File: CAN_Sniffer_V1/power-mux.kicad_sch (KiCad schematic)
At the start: 7 parts, among them IC1 TPS2121RUXR

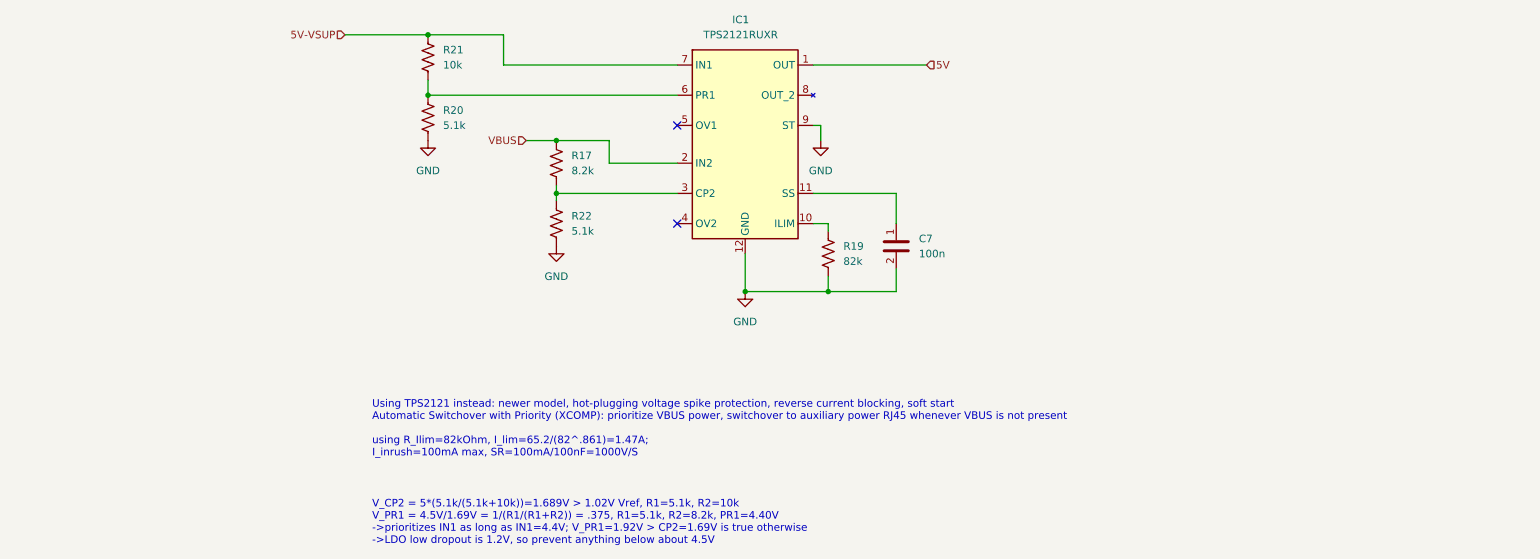
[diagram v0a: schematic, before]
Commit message: iteration 2 routing
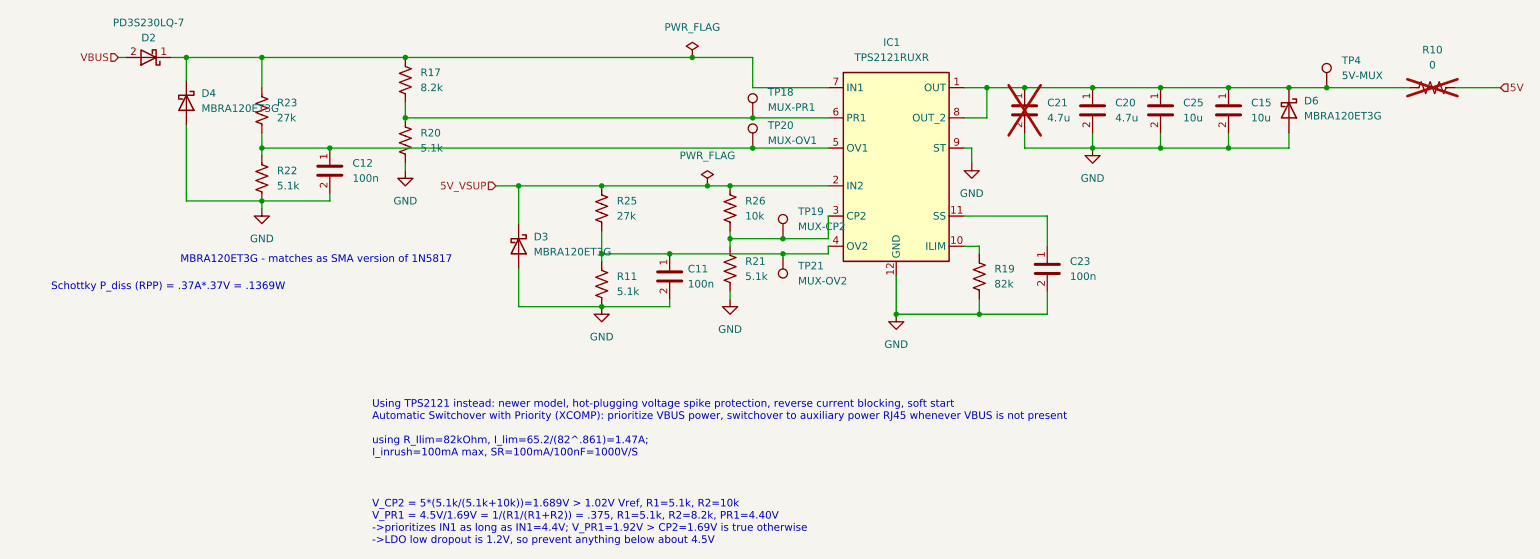
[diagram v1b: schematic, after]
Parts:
- removed C7: 100n, Capacitor_SMD:C_0402_1005Metric_Pad0.74x0.62mm_HandSolder, symbol bfr_capacitors:CL05B104KB54PNC
- removed R20, R22: 5.1k, Resistor_SMD:R_0402_1005Metric_Pad0.72x0.64mm_HandSolder, symbol bfr_resistors:RMCF0402FT5K10
- removed R21: 10k, Resistor_SMD:R_0402_1005Metric_Pad0.72x0.64mm_HandSolder, symbol bfr_resistors:RMCF0402FT10K0
- added C11, C12: 100n, Capacitor_SMD:C_0402_1005Metric_Pad0.74x0.62mm_HandSolder, symbol bfr_capacitors:CL05B104KB54PNC
- added C15, C25: 10u, Capacitor_SMD:C_0603_1608Metric_Pad1.08x0.95mm_HandSolder, symbol bfr_capacitors:CL10A106MA8NRNC
- added C20, C21: 4.7u, Capacitor_SMD:C_0603_1608Metric_Pad1.08x0.95mm_HandSolder, symbol bfr_capacitors:CL10A475KO8NNNC
- added C23: 100n, Capacitor_SMD:C_0603_1608Metric_Pad1.08x0.95mm_HandSolder, symbol bfr_capacitors:06035C104KAT2A
- added D2: PD3S230LQ-7, PD3S230LQ-7:PD3S230LQ7, symbol PD3S230LQ-7:PD3S230LQ-7
- added D3, D4, D6: MBRA120ET3G, Diode_SMD:D_SMA_Handsoldering, symbol Diode:1N5817
- added R10: 0, Resistor_SMD:R_0805_2012Metric_Pad1.20x1.40mm_HandSolder, symbol bfr_resistors:RMCF0805ZT0R00
- added R11, R20, R21, R22: 5.1k, Resistor_SMD:R_0603_1608Metric_Pad0.98x0.95mm_HandSolder, symbol bfr_resistors:RMCF0603FT5K10
- added R23, R25: 27k, Resistor_SMD:R_0603_1608Metric_Pad0.98x0.95mm_HandSolder, symbol bfr_resistors:RMCF0603FT27K0
- added R26: 10k, Resistor_SMD:R_0603_1608Metric_Pad0.98x0.95mm_HandSolder, symbol bfr_resistors:RMCF0603FT10K0
- added TP18: MUX-PR1, TestPoint:TestPoint_Pad_D1.0mm, symbol Connector:TestPoint
- added TP19: MUX-CP2, TestPoint:TestPoint_Pad_D1.0mm, symbol Connector:TestPoint
- added TP20: MUX-OV1, TestPoint:TestPoint_Pad_D1.0mm, symbol Connector:TestPoint
- added TP21: MUX-OV2, TestPoint:TestPoint_Pad_D1.0mm, symbol Connector:TestPoint
- added TP4: 5V-MUX, TestPoint:TestPoint_Pad_D1.0mm, symbol Connector:TestPoint
- IC1: JLC link (none) -> https://jlcpcb.com/partdetail/TexasInstruments-TPS2121RUXR/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
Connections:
- net 5V: now also R10.2; no longer IC1.1 (OUT)
- net GND: now also C11.2, C12.2, C15.2, C20.2, C21.2, C23.2, C25.2, D3.2 (A), D4.2 (A), D6.2 (A), R11.1, R20.1, R21.1, R22.1
- net VBUS: now also D2.2 (A); no longer IC1.2 (IN2), R17.2
- net at IC1.11 (SS): now also C23.1
- net at IC1.3 (CP2): now also R21.2, R26.1, TP19.1; no longer R17.1
- net at IC1.4 (OV2): now also C11.1, R11.2, R25.1, TP21.1
- net at IC1.5 (OV1): now also C12.1, R22.2, R23.1, TP20.1
- net at IC1.6 (PR1): now also R17.1, R20.2, TP18.1
- net at IC1.8 (OUT_2): now also IC1.1 (OUT), C15.1, C20.1, C21.1, C25.1, D6.1 (K), R10.1, TP4.1
- net 5V-VSUP: no longer names the net of IC1.7 (IN1)
- net 5V-VSUP: now also R17.2, D2.1 (K), D4.1 (K), R23.2
- new net 5V_VSUP: D3.1 (K), IC1.2 (IN2), R25.2, R26.2
- no-connect marks 2 -> 0
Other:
- note added: "MBRA120ET3G - matches as SMA version of 1N5817"
- note added: "Schottky P_diss (RPP) = .37A*.37V = .1369W"
- moved on the sheet: R17, R19

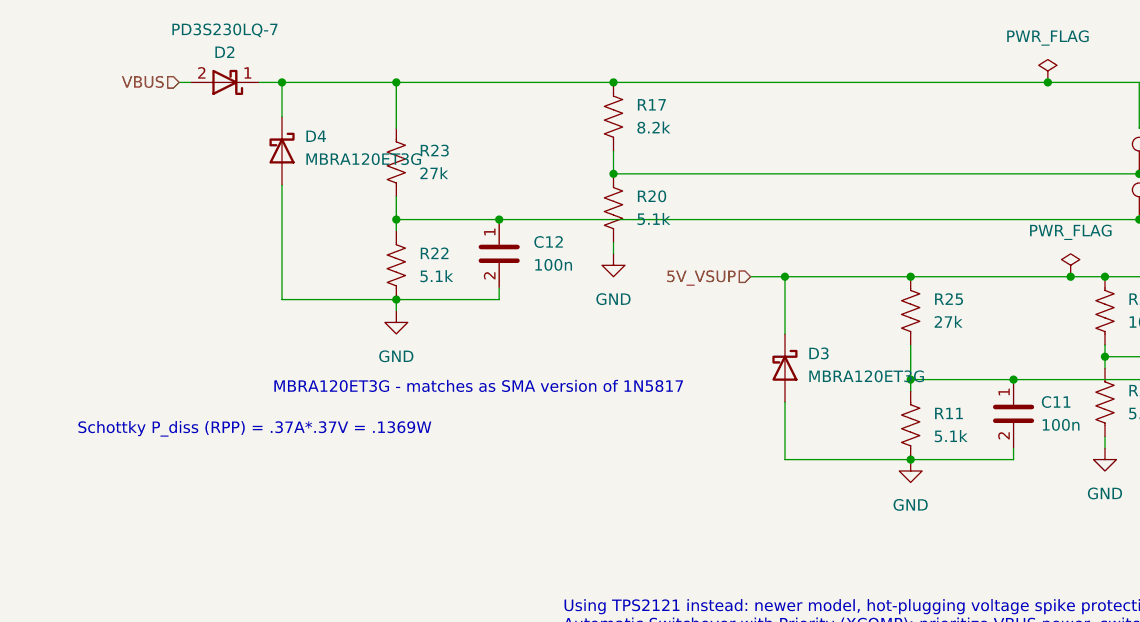
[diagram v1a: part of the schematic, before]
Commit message: sync changes
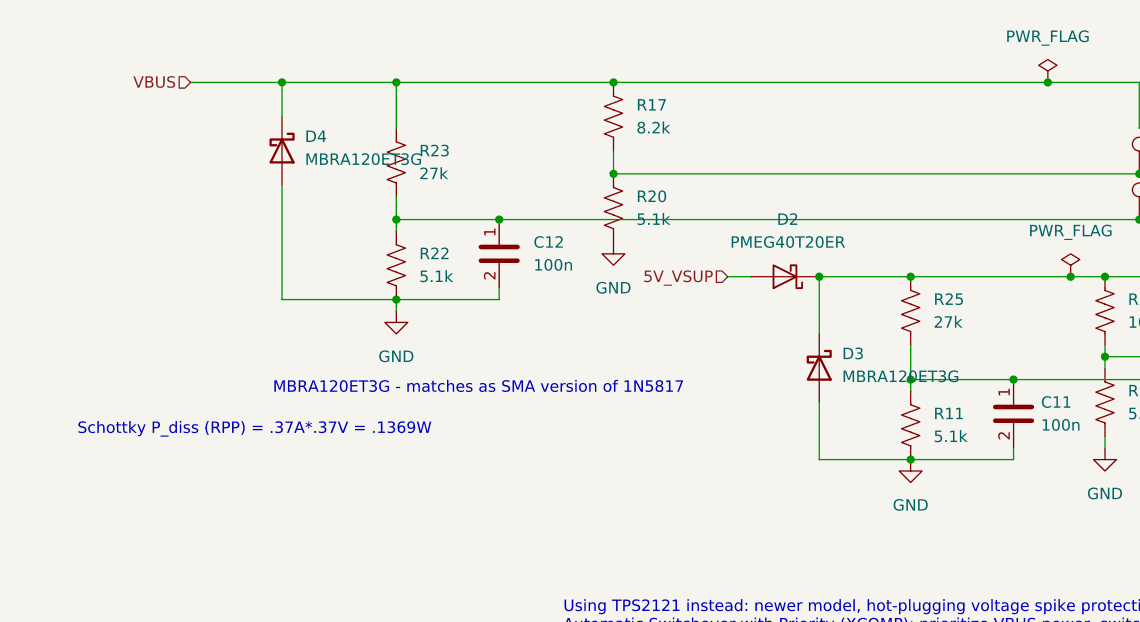
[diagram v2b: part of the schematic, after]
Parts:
- removed D2: PD3S230LQ-7, PD3S230LQ-7:PD3S230LQ7, symbol PD3S230LQ-7:PD3S230LQ-7
- added D2: PMEG40T20ER, Diode_SMD:Nexperia_CFP3_SOD-123W, symbol Diode:PMEG40T20ER
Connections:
- net 5V_VSUP: now also D2.2 (A); no longer D3.1 (K), IC1.2 (IN2), R25.2, R26.2
- net VBUS: now also D4.1 (K), IC1.7 (IN1), R17.2, R23.2
- new net: D2.1 (K), D3.1 (K), IC1.2 (IN2), R25.2, R26.2
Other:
- moved on the sheet: D3
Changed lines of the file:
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@@
 	)
 	(junction
+		(at 105.41 83.82)
+		(diameter 0)
+		(color 0 0 0 0)
+	)
+	(junction
 		(at 180.34 67.31)
 		(diameter 0)
@@
 	)
 	(junction
-		(at 101.6 83.82)
-		(diameter 0)
-		(color 0 0 0 0)
-	)
-	(junction
 		(at 69.85 77.47)
 		(diameter 0)
@@
 	(wire
 		(pts
-			(xy 43.18 62.23) (xy 45.72 62.23)
-		)
-		(stroke
-			(width 0)
-			(type default)
-		)
-	)
-	(wire
-		(pts
 			(xy 130.81 62.23) (xy 140.97 62.23)
 		)
@@
 	(wire
 		(pts
-			(xy 101.6 83.82) (xy 101.6 90.17)
+			(xy 105.41 83.82) (xy 105.41 90.17)
 		)
 		(stroke
@@
 	(wire
 		(pts
-			(xy 82.55 81.28) (xy 82.55 80.01)
-		)
-		(stroke
-			(width 0)
-			(type default)
-		)
-	)
-	(wire
-		(pts
 			(xy 82.55 62.23) (xy 130.81 62.23)
 		)
@@
 	(wire
 		(pts
-			(xy 101.6 104.14) (xy 115.57 104.14)
+			(xy 105.41 104.14) (xy 115.57 104.14)
 		)
 		(stroke
@@
 	(wire
 		(pts
-			(xy 101.6 97.79) (xy 101.6 104.14)
+			(xy 105.41 97.79) (xy 105.41 104.14)
 		)
 		(stroke
@@
 	(wire
 		(pts
-			(xy 101.6 83.82) (xy 115.57 83.82)
-		)
-		(stroke
-			(width 0)
-			(type default)
-		)
-	)
-	(wire
-		(pts
 			(xy 179.07 105.41) (xy 179.07 102.87)
 		)
@@
 	(wire
 		(pts
-			(xy 97.79 83.82) (xy 101.6 83.82)
+			(xy 95.25 83.82) (xy 97.79 83.82)
 		)
 		(stroke
@@
 	(wire
 		(pts
-			(xy 34.29 62.23) (xy 35.56 62.23)
+			(xy 35.56 62.23) (xy 45.72 62.23)
 		)
 		(stroke
@@
 	(wire
 		(pts
+			(xy 105.41 83.82) (xy 115.57 83.82)
+		)
+		(stroke
+			(width 0)
+			(type default)
+		)
+	)
+	(wire
+		(pts
 			(xy 140.97 67.31) (xy 153.67 67.31)
 		)
@@
 	(hierarchical_label "5V_VSUP"
 		(shape input)
-		(at 97.79 83.82 180)
+		(at 95.25 83.82 180)
 		(effects
 			(font
@@
 	(hierarchical_label "VBUS"
 		(shape input)
-		(at 34.29 62.23 180)
+		(at 35.56 62.23 180)
 		(effects
 			(font
@@
 	(symbol
 		(lib_id "Diode:1N5817")
-		(at 101.6 93.98 270)
+		(at 105.41 93.98 270)
 		(unit 1)
 		(exclude_from_sim no)
@@
 		(fields_autoplaced yes)
 		(property "Reference" "D3"
-			(at 104.14 92.3924 90)
+			(at 107.95 92.3924 90)
 			(effects
 				(font
@@
 		)
 		(property "Value" "MBRA120ET3G"
-			(at 104.14 94.9324 90)
+			(at 107.95 94.9324 90)
 			(effects
 				(font
@@
 		)
 		(property "Footprint" "Diode_SMD:D_SMA_Handsoldering"
-			(at 97.155 93.98 0)
+			(at 100.965 93.98 0)
 			(effects
 				(font
@@
 		)
 		(property "Datasheet" "https://www.onsemi.com/pdf/datasheet/mbra120et3-d.pdf"
-			(at 101.6 93.98 0)
+			(at 105.41 93.98 0)
 			(effects
 				(font
@@
 		)
 		(property "Description" "DIODE SCHOTTKY 20V 1A SMA"
-			(at 101.6 93.98 0)
+			(at 105.41 93.98 0)
 			(effects
 				(font
@@
 		)
 		(property "Mouser PN" "MBRA120ET3G"
-			(at 101.6 93.98 90)
+			(at 105.41 93.98 90)
 			(effects
 				(font
@@
 		)
 		(property "Mouser link" "https://www.mouser.com/ProductDetail/onsemi/MBRA120ET3G?qs=3JMERSakebpxyEF0miqDLQ%3D%3D&srsltid=AfmBOorHUs3U0aY5FgYfyQY2nJZMbm20r44N94gas6_FtPkWxmMa-o96"
-			(at 101.6 93.98 90)
+			(at 105.41 93.98 90)
 			(effects
 				(font
@@
 		)
 		(property "Digikey PN" "MBRA120ET3G"
-			(at 101.6 93.98 90)
+			(at 105.41 93.98 90)
 			(effects
 				(font
@@
 		)
 		(property "Digikey link" "https://www.digikey.com/en/products/detail/onsemi/MBRA120ET3G/920609"
-			(at 101.6 93.98 90)
+			(at 105.41 93.98 90)
 			(effects
 				(font
@@
 	)
 	(symbol
-		(lib_id "PD3S230LQ-7:PD3S230LQ-7")
-		(at 43.18 62.23 180)
-		(unit 1)
-		(exclude_from_sim no)
-		(in_bom yes)
-		(on_board yes)
-		(dnp no)
-		(property "Reference" "D2"
-			(at 39.37 58.928 0)
-			(effects
-				(font
-					(size 1.27 1.27)
-				)
-			)
-		)
-		(property "Value" "PD3S230LQ-7"
-			(at 39.37 56.388 0)
-			(effects
-				(font
-					(size 1.27 1.27)
-				)
-			)
-		)
-		(property "Footprint" "PD3S230LQ-7:PD3S230LQ7"
-			(at 30.48 -31.42 0)
-			(effects
-				(font
-					(size 1.27 1.27)
-				)
-				(justify left top)
-				(hide yes)
-			)
-		)
-		(property "Datasheet" "https://www.diodes.com/assets/Datasheets/ds31751.pdf"
-			(at 30.48 -131.42 0)
-			(effects
-				(font
-					(size 1.27 1.27)
-				)
-				(justify left top)
-				(hide yes)
-			)
-		)
-		(property "Description" "Schottky Diode 30 V 2A Surface Mount PowerDI 323"
-			(at 43.18 62.23 0)
-			(effects
-				(font
-					(size 1.27 1.27)
-				)
-				(hide yes)
-			)
-		)
-		(property "Height" "0.7"
-			(at 30.48 -331.42 0)
-			(effects
-				(font
-					(size 1.27 1.27)
-				)
-				(justify left top)
-				(hide yes)
-			)
-		)
-		(property "Mouser Part Number" "621-PD3S230LQ-7"
-			(at 30.48 -431.42 0)
-			(effects
-				(font
-					(size 1.27 1.27)
-				)
-				(justify left top)
-				(hide yes)
-			)
-		)
-		(property "Mouser Price/Stock" "https://www.mouser.co.uk/ProductDetail/Diodes-Incorporated/PD3S230LQ-7?qs=vdQOMtKMWaDhkf1xtelm%2FA%3D%3D"
-			(at 30.48 -531.42 0)
-			(effects
-				(font
-					(size 1.27 1.27)
-				)
-				(justify left top)
-				(hide yes)
-			)
-		)
-		(property "Manufacturer_Name" "Diodes Incorporated"
-			(at 30.48 -631.42 0)
-			(effects
-				(font
-					(size 1.27 1.27)
-				)
-				(justify left top)
-				(hide yes)
-			)
-		)
-		(property "Manufacturer_Part_Number" "PD3S230LQ-7"
-			(at 30.48 -731.42 0)
-			(effects
-				(font
-					(size 1.27 1.27)
-				)
-				(justify left top)
-				(hide yes)
-			)
-		)
-		(property "Mouser link" "https://www.mouser.com/ProductDetail/Diodes-Incorporated/PD3S230LQ-7?qs=vdQOMtKMWaDhkf1xtelm%2FA%3D%3D"
-			(at 43.18 62.23 0)
-			(effects
-				(font
-					(size 1.27 1.27)
-				)
-				(hide yes)
-			)
-		)
-		(property "Digikey link" "https://www.digikey.com/en/products/detail/diodes-incorporated/PD3S230LQ-7/4868784"
-			(at 43.18 62.23 0)
-			(effects
-				(font
-					(size 1.27 1.27)
-				)
-				(hide yes)
-			)
-		)
-		(pin "2"
-		)
-		(pin "1"
-		)
-		(instances
-			(project "CAN_Sniffer_1.0"
-				(path "/e451ff56-2618-4e84-9d3d-2972ad7496ed/a595fcef-79dc-47ac-8894-f92a4a37cf31/11984be6-3055-47d4-aea0-5eeba7b3bd2c"
-					(reference "D2")
-					(unit 1)
-				)
-			)
-		)
-	)
-	(symbol
 		(lib_id "power:GND")
-		(at 82.55 81.28 0)
+		(at 82.55 80.01 0)
 		(unit 1)
 		(exclude_from_sim no)
@@
 		(fields_autoplaced yes)
 		(property "Reference" "#PWR027"
-			(at 82.55 87.63 0)
+			(at 82.55 86.36 0)
 			(effects
 				(font
@@
 		)
 		(property "Value" "GND"
-			(at 82.55 86.36 0)
+			(at 82.55 85.09 0)
 			(effects
 				(font
@@
 		)
 		(property "Footprint" ""
-			(at 82.55 81.28 0)
+			(at 82.55 80.01 0)
 			(effects
 				(font
@@
 		)
 		(property "Datasheet" ""
-			(at 82.55 81.28 0)
+			(at 82.55 80.01 0)
 			(effects
 				(font
@@
 		)
 		(property "Description" "Power symbol creates a global label with name \"GND\" , ground"
-			(at 82.55 81.28 0)
+			(at 82.55 80.01 0)
 			(effects
 				(font
@@
 					(unit 1)
 				)
+			)
+		)
+	)
+	(symbol
+		(lib_id "Diode:PMEG40T20ER")
+		(at 101.6 83.82 180)
+		(unit 1)
+		(exclude_from_sim no)
+		(in_bom yes)
+		(on_board yes)
+		(dnp no)
+		(fields_autoplaced yes)
+		(property "Reference" "D2"
+			(at 101.9175 77.47 0)
+			(effects
+				(font
+					(size 1.27 1.27)
+				)
+			)
+		)
+		(property "Value" "PMEG40T20ER"
+			(at 101.9175 80.01 0)
+			(effects
+				(font
+					(size 1.27 1.27)
+				)
+			)
+		)
+		(property "Footprint" "Diode_SMD:Nexperia_CFP3_SOD-123W"
+			(at 101.6 79.375 0)
+			(effects
+				(font
+					(size 1.27 1.27)
+				)
+				(hide yes)
+			)
+		)
+		(property "Datasheet" "https://assets.nexperia.com/documents/data-sheet/PMEG40T20ER.pdf"
+			(at 101.6 83.82 0)
+			(effects
+				(font
+					(size 1.27 1.27)
+				)
+				(hide yes)
+			)
+		)
+		(property "Description" "40V, 2A low Vf Trench MEGA Schottky barrier rectifier, SOD-123W"
+			(at 101.6 83.82 0)
+			(effects
+				(font
+					(size 1.27 1.27)
+				)
+				(hide yes)
+			)
+		)
+		(pin "1"
+		)
+		(pin "2"
+		)
+		(instances
+			(project ""
+				(path "/e451ff56-2618-4e84-9d3d-2972ad7496ed/a595fcef-79dc-47ac-8894-f92a4a37cf31/11984be6-3055-47d4-aea0-5eeba7b3bd2c"
+					(reference "D2")
+					(unit 1)
+				)
